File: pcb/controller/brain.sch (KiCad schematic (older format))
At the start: 0 parts

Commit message: designed v0.1 of brain board
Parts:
- added C1, C2, C3, C4, C5: 1uF, Capacitors_SMD:C_0603_HandSoldering, symbol C
- added GND1, Mode1, RX1, Reset1, TX1: TP, Measurement_Points:Measurement_Point_Round-SMD-Pad_Small, symbol TEST
- added J1: CONN_02X08, Pin_Headers:Pin_Header_Straight_2x08_Pitch2.54mm_SMD, symbol CONN_02X08
- added J10, J11, J12, J13, J14, J15, J16, J17, J18, J19, J20, J21, J22, J23, J24, J25, J26, J27, J28, J29, J30, J31, J32, J33, J34, J35, J36, J37, J38, J39, J40, J41, J42, J43, J44, J45, J46, J5, J6, J7, J8, J9: break, breakaway:0.35mil_square, symbol TEST_1P
- added J2, J3, J4: CONN_01X08, Pin_Headers:Pin_Header_Straight_1x08_Pitch2.54mm_SMD_Pin1Right, symbol CONN_01X08
- added J47, J48, J49: CONN_01X01, SMD_Packages:1Pin, symbol CONN_01X01
- added Q1, Q10, Q11, Q12, Q13, Q14, Q15, Q16, Q17, Q18, Q19, Q2, Q20, Q21, Q22, Q23, Q24, Q25, Q26, Q27, Q28, Q29, Q3, Q30, Q31, Q32, Q4, Q5, Q6, Q7, Q8, Q9: A09T, TO_SOT_Packages_SMD:SOT-23, symbol Q_NMOS_GSD
- added R1, R2: 1k, Resistors_SMD:R_0603_HandSoldering, symbol R
- added U1, U2, U3, U4: 74HC595, Housings_SOIC:SOIC-16_3.9x9.9mm_Pitch1.27mm, symbol 74HC595
- added U5: ESP-12E, ESP8266:ESP-12E_SMD, symbol ESP-12E
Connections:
- new net: R1.1, Reset1.1, U5.1 (REST)
- new net: Mode1.1, R2.1, U5.12 (GPIO0)
- new net: RX1.1, U5.15 (RXD)
- new net: TX1.1, U5.16 (TXD)
- new net: Q10.1 (G), U2.1 (QB)
- new net: Q9.1 (G), U2.15 (QA)
- new net: Q11.1 (G), U2.2 (QC)
- new net: Q12.1 (G), U2.3 (QD)
- new net: Q13.1 (G), U2.4 (QE)
- new net: Q14.1 (G), U2.5 (QF)
- new net: Q15.1 (G), U2.6 (QG)
- new net: Q16.1 (G), U2.7 (QH)
- new net: J21.1, J22.1, U2.9 (~QH), U3.14 (SER)
- new net: Q18.1 (G), U3.1 (QB)
- new net: Q17.1 (G), U3.15 (QA)
- new net: Q19.1 (G), U3.2 (QC)
- new net: Q20.1 (G), U3.3 (QD)
- new net: Q21.1 (G), U3.4 (QE)
- new net: Q22.1 (G), U3.5 (QF)
- new net: Q23.1 (G), U3.6 (QG)
- new net: Q24.1 (G), U3.7 (QH)
- new net: J33.1, J34.1, U3.9 (~QH), U4.14 (SER)
- new net: Q26.1 (G), U4.1 (QB)
- new net: Q25.1 (G), U4.15 (QA)
- new net: Q27.1 (G), U4.2 (QC)
- new net: Q28.1 (G), U4.3 (QD)
- new net: Q29.1 (G), U4.4 (QE)
- new net: Q30.1 (G), U4.5 (QF)
- new net: Q31.1 (G), U4.6 (QG)
- new net: Q32.1 (G), U4.7 (QH)
- new net: J43.1, U4.9 (~QH)
- new net: Q2.1 (G), U1.1 (QB)
- new net: Q1.1 (G), U1.15 (QA)
- new net: Q3.1 (G), U1.2 (QC)
- new net: Q4.1 (G), U1.3 (QD)
- new net: Q5.1 (G), U1.4 (QE)
- new net: Q6.1 (G), U1.5 (QF)
- new net: Q7.1 (G), U1.6 (QG)
- new net: Q8.1 (G), U1.7 (QH)
- new net +12V: J1.1 (P1), J1.2 (P2), J47.1 (P1)
- new net ADC_RCLK: J11.1, J12.1, J23.1, J24.1, J35.1, J36.1, J44.1, U2.12 (RCLK), U3.12 (RCLK), U4.12 (RCLK), U5.6 (GPIO12)
- new net CLK: J1.7 (P7), J13.1, J14.1, J25.1, J26.1, J37.1, J38.1, J45.1, U1.11 (SRCLK), U2.11 (SRCLK), U3.11 (SRCLK), U4.11 (SRCLK), U5.22 (SCLK)
- new net GND: C1.1, C2.1, C3.1, C4.1, C5.1, GND1.1, J1.3 (P3), J1.4 (P4), J15.1, J16.1, J19.1, J20.1, J27.1, J28.1, J31.1, J32.1, J39.1, J40.1, J42.1, J46.1, J49.1 (P1), J7.1, J8.1, Q1.2 (S), Q10.2 (S), Q11.2 (S), Q12.2 (S), Q13.2 (S), Q14.2 (S), Q15.2 (S), Q16.2 (S), Q17.2 (S), Q18.2 (S), Q19.2 (S), Q2.2 (S), Q20.2 (S), Q21.2 (S), Q22.2 (S), Q23.2 (S), Q24.2 (S), Q25.2 (S), Q26.2 (S), Q27.2 (S), Q28.2 (S), Q29.2 (S), Q3.2 (S), Q30.2 (S), Q31.2 (S), Q32.2 (S), Q4.2 (S), Q5.2 (S), Q6.2 (S), Q7.2 (S), Q8.2 (S), Q9.2 (S), U1.13 (G), U1.8 (GND), U2.13 (G), U2.8 (GND), U3.13 (G), U3.8 (GND), U4.13 (G), U4.8 (GND)
- new net MISO: J1.6 (P6), U5.18 (MISO)
- new net MOSI: J10.1, J9.1, U1.14 (SER), U2.14 (SER), U5.21 (MOSI)
- new net N_ADC0: J2.1 (P1), Q9.3 (D)
- new net N_ADC1: J2.2 (P2), Q10.3 (D)
- new net N_ADC10: J3.3 (P3), Q19.3 (D)
- new net N_ADC11: J3.4 (P4), Q20.3 (D)
- new net N_ADC12: J3.5 (P5), Q21.3 (D)
- new net N_ADC13: J3.6 (P6), Q22.3 (D)
- new net N_ADC14: J3.7 (P7), Q23.3 (D)
- new net N_ADC15: J3.8 (P8), Q24.3 (D)
- new net N_ADC16: J4.1 (P1), Q25.3 (D)
- new net N_ADC17: J4.2 (P2), Q26.3 (D)
- new net N_ADC18: J4.3 (P3), Q27.3 (D)
- new net N_ADC19: J4.4 (P4), Q28.3 (D)
- new net N_ADC2: J2.3 (P3), Q11.3 (D)
- new net N_ADC20: J4.5 (P5), Q29.3 (D)
- new net N_ADC21: J4.6 (P6), Q30.3 (D)
- new net N_ADC22: J4.7 (P7), Q31.3 (D)
- new net N_ADC23: J4.8 (P8), Q32.3 (D)
- new net N_ADC3: J2.4 (P4), Q12.3 (D)
- new net N_ADC4: J2.5 (P5), Q13.3 (D)
- new net N_ADC5: J2.6 (P6), Q14.3 (D)
- new net N_ADC6: J2.7 (P7), Q15.3 (D)
- new net N_ADC7: J2.8 (P8), Q16.3 (D)
- new net N_ADC8: J3.1 (P1), Q17.3 (D)
- new net N_ADC9: J3.2 (P2), Q18.3 (D)
- new net N_LOAD: J1.8 (P8), U5.10 (GPIO15)
- new net N_START0: J1.9 (P9), Q1.3 (D)
- new net N_START1: J1.10 (P10), Q2.3 (D)
- new net N_START2: J1.11 (P11), Q3.3 (D)
- new net N_START3: J1.12 (P12), Q4.3 (D)
- new net N_START4: J1.13 (P13), Q5.3 (D)
- new net N_START5: J1.14 (P14), Q6.3 (D)
- new net N_START6: J1.15 (P15), Q7.3 (D)
- new net N_START7: J1.16 (P16), Q8.3 (D)
- new net START_RCLK: U1.12 (RCLK), U5.7 (GPIO13)
- new net VCC: C1.2, C2.2, C3.2, C4.2, C5.2, J1.5 (P5), J17.1, J18.1, J29.1, J30.1, J41.1, J48.1 (P1), J5.1, J6.1, R1.2, R2.2, U1.10 (SRCLR), U1.16 (VCC), U2.10 (SRCLR), U2.16 (VCC), U3.10 (SRCLR), U3.16 (VCC), U4.10 (SRCLR), U4.16 (VCC)
- no-connect marks 0 -> 13

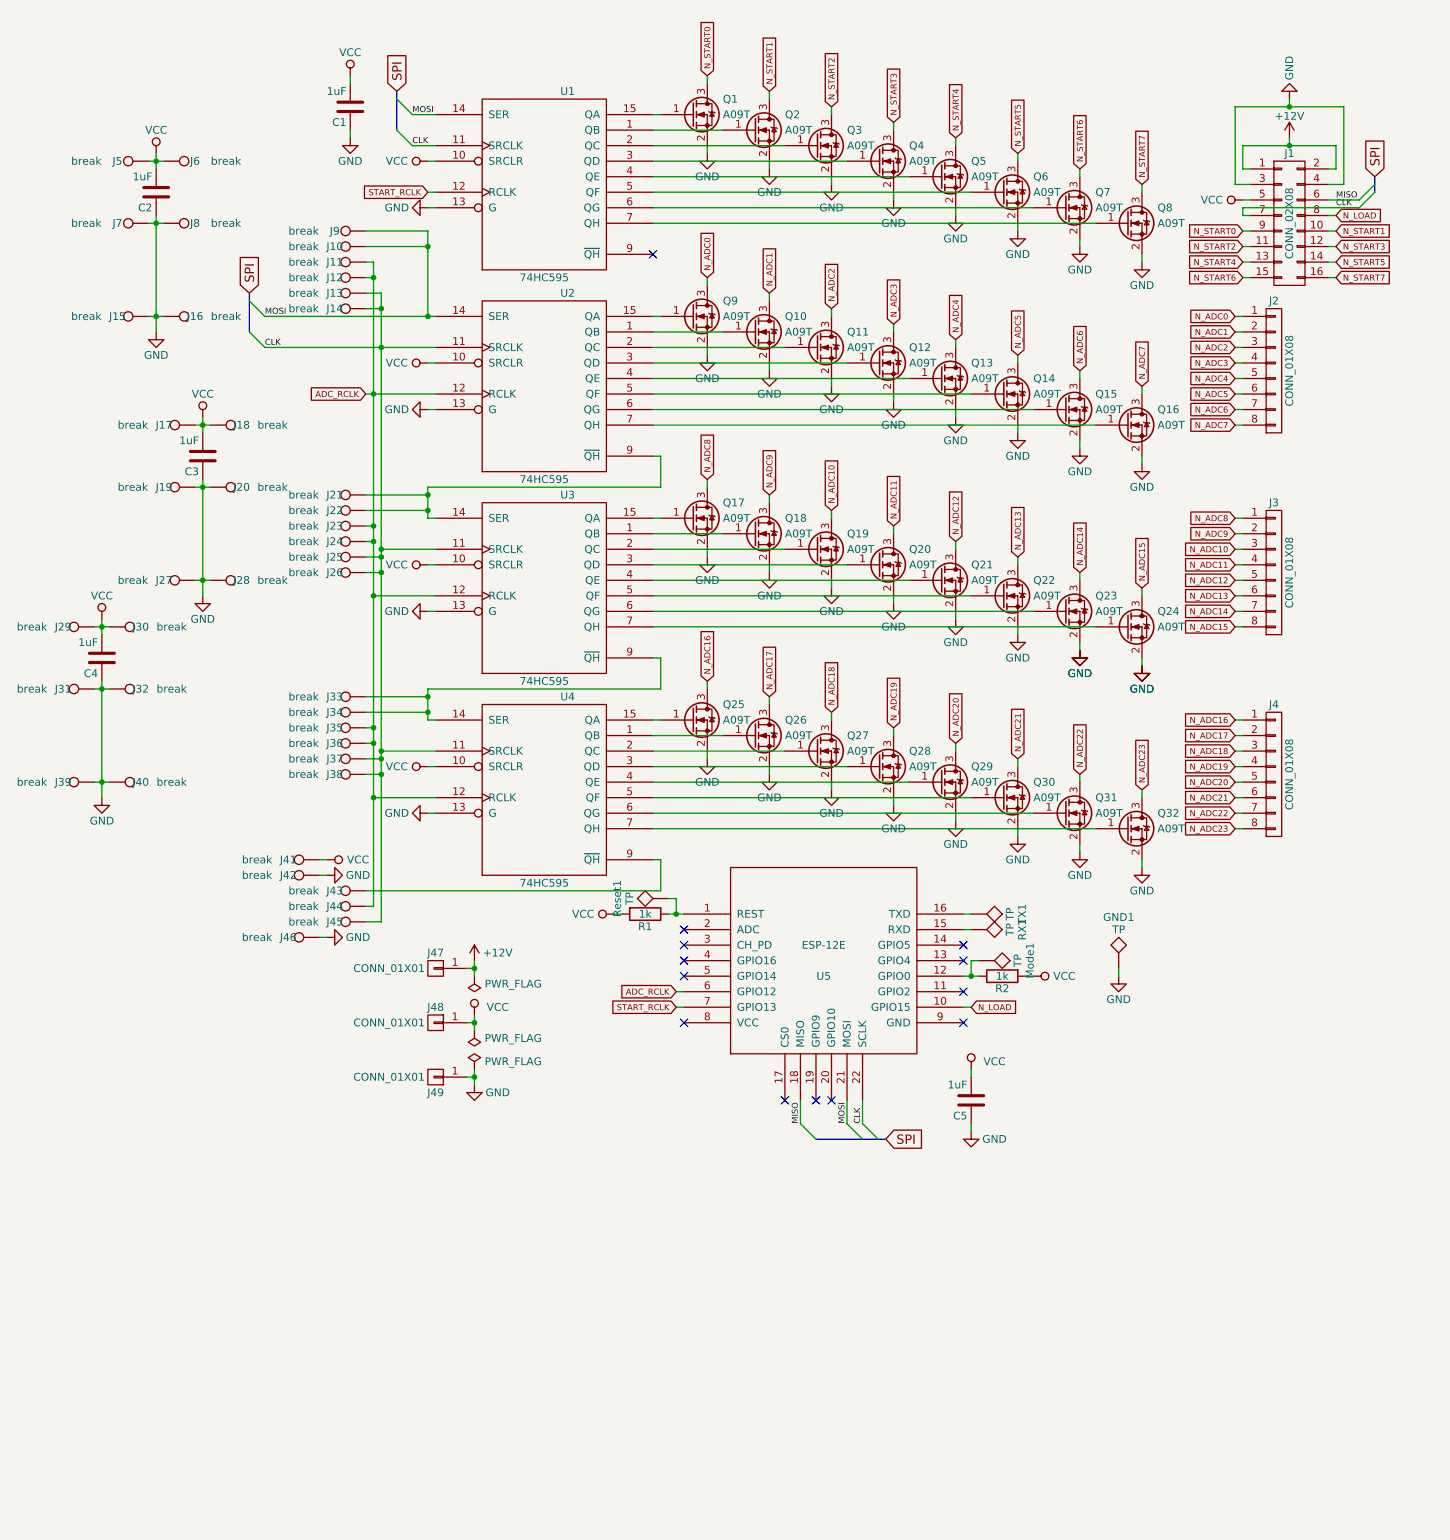
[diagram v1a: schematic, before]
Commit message: begins to further develop controller
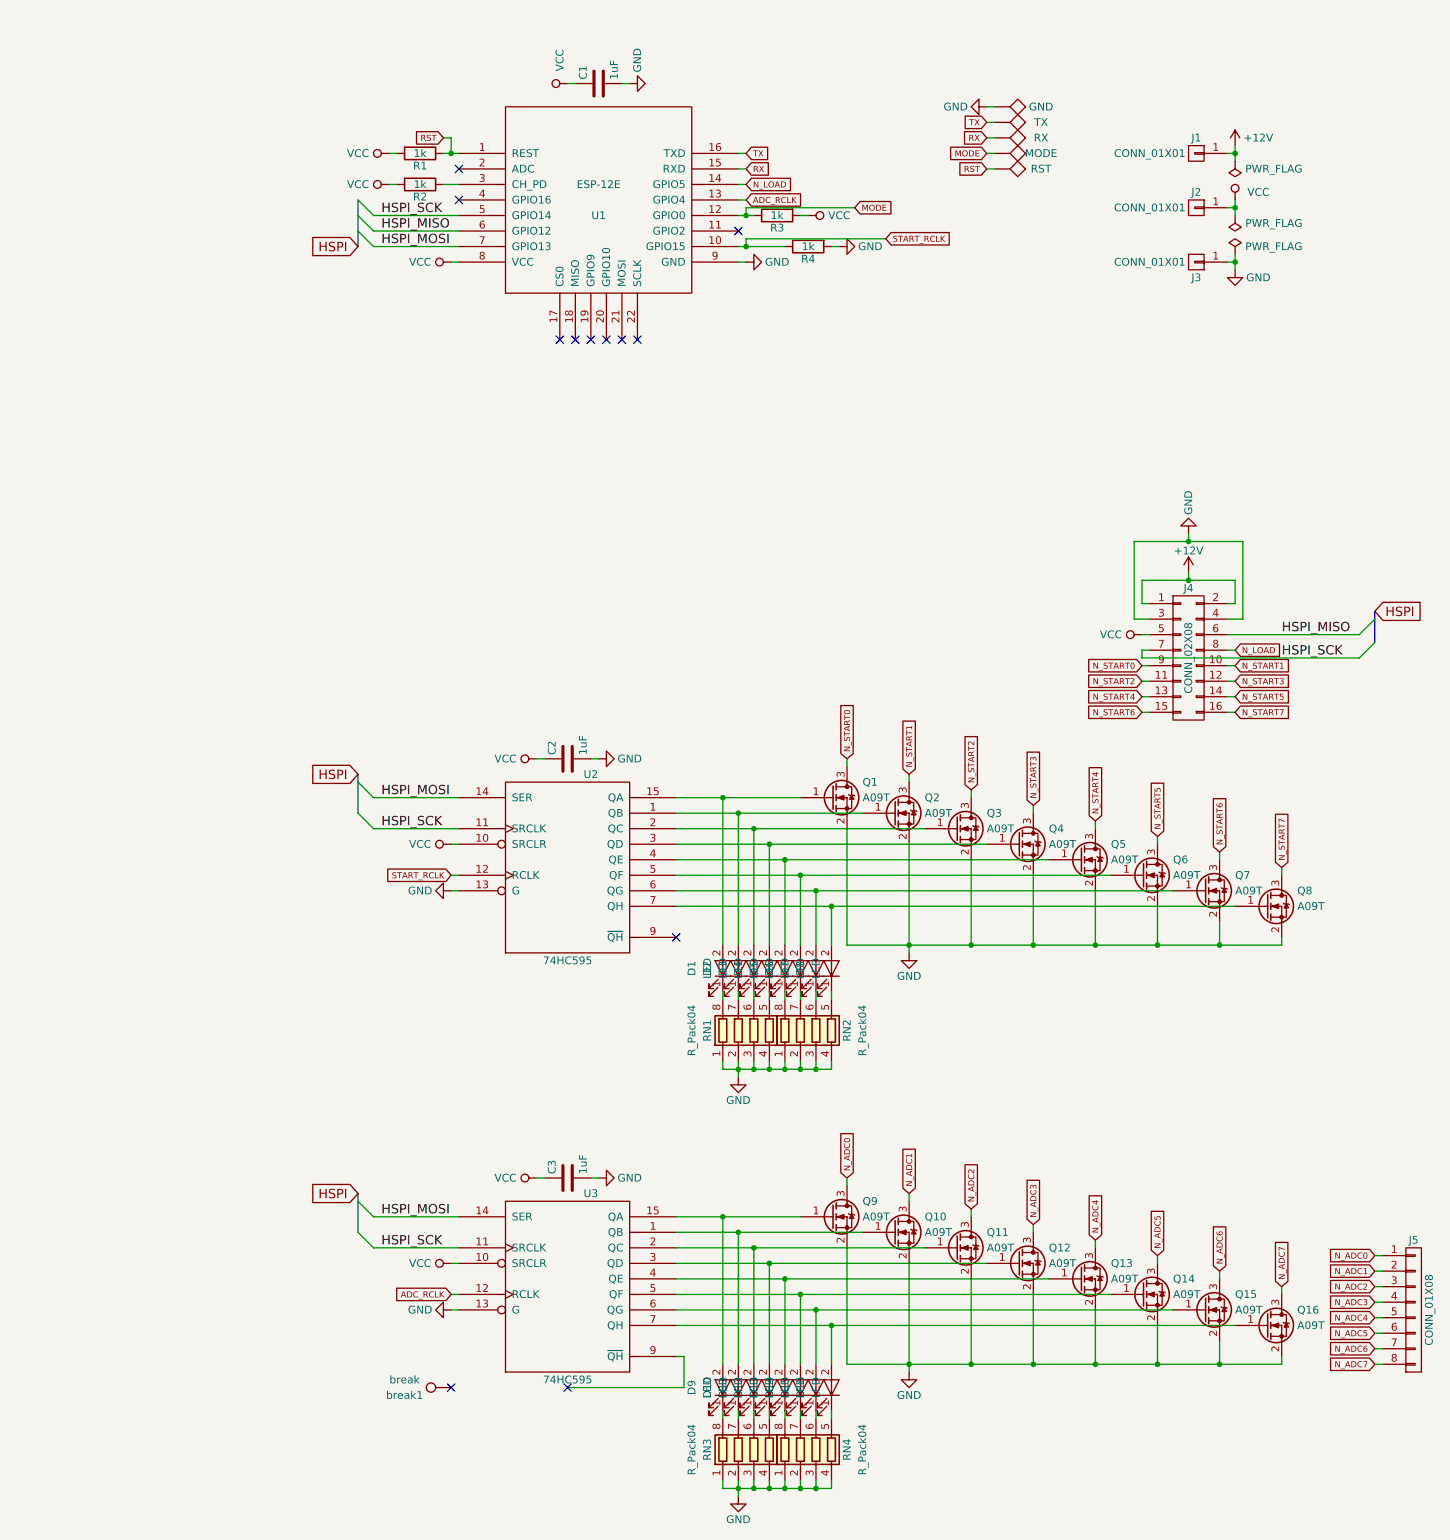
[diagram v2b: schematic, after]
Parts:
- removed C2, C4: 1uF, Capacitors_SMD:C_0603_HandSoldering, symbol C
- removed J10, J11, J12, J13, J14, J15, J16, J17, J18, J19, J20, J21, J22, J23, J24, J25, J26, J27, J28, J29, J30, J31, J32, J33, J34, J35, J36, J37, J38, J39, J40, J41, J42, J43, J44, J45, J46, J5, J6, J7, J8, J9: break, breakaway:0.35mil_square, symbol TEST_1P
- removed J3, J4: CONN_01X08, Pin_Headers:Pin_Header_Straight_1x08_Pitch2.54mm_SMD_Pin1Right, symbol CONN_01X08
- removed Q17, Q18, Q19, Q20, Q21, Q22, Q23, Q24, Q25, Q26, Q27, Q28, Q29, Q30, Q31, Q32: A09T, TO_SOT_Packages_SMD:SOT-23, symbol Q_NMOS_GSD
- removed U2, U4: 74HC595, Housings_SOIC:SOIC-16_3.9x9.9mm_Pitch1.27mm, symbol 74HC595
- added D1, D10, D11, D12, D13, D14, D15, D16, D2, D3, D4, D5, D6, D7, D8, D9: LED, LEDs:LED_0603, symbol LED
- added R2, R4: 1k, Resistors_SMD:R_0603_HandSoldering, symbol R
- added RN1, RN2, RN3, RN4: R_Pack04, Resistors_SMD:R_Array_Convex_4x0603, symbol R_Pack04
- added break1: break, symbol TEST_1P
- J4: renamed from J1; footprint Pin_Headers:Pin_Header_Straight_2x08_Pitch2.54mm_SMD -> Connectors:IDC_Header_SMD_16pins
- TP1: renamed from GND1; value TP -> GND
- TP2: renamed from TX1; value TP -> TX
- TP3: renamed from RX1; value TP -> RX
- TP4: renamed from Mode1; value TP -> MODE
- TP5: renamed from Reset1; value TP -> RST
- renumbered C5 to C1, C1 to C2, J47 to J1, J48 to J2, J49 to J3, J2 to J5, R2 to R3, U5 to U1, U1 to U2
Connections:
- net ADC_RCLK: now also U1.13 (GPIO4); no longer U1.6 (GPIO12)
- net GND: now also C1.2, C2.2, C3.2, U1.9 (GND), R4.2, RN1.1 (R1.1), RN1.2 (R2.1), RN1.3 (R3.1), RN1.4 (R4.1), RN2.1 (R1.1), RN2.2 (R2.1), RN2.3 (R3.1), RN2.4 (R4.1), RN3.1 (R1.1), RN3.2 (R2.1), RN3.3 (R3.1), RN3.4 (R4.1), RN4.1 (R1.1), RN4.2 (R2.1), RN4.3 (R3.1), RN4.4 (R4.1); no longer C1.1, C2.1, C3.1
- net N_LOAD: now also U1.14 (GPIO5); no longer U1.10 (GPIO15)
- net START_RCLK: now also U1.10 (GPIO15), R4.1; no longer U1.7 (GPIO13)
- net VCC: now also C1.1, C2.1, C3.1, U1.8 (VCC), R2.2; no longer C1.2, C2.2, C3.2
- net RST: now reaches R1.1, TP5.1, U1.1 (REST)
- net MODE: now reaches R3.1, TP4.1, U1.12 (GPIO0)
- net RX: now reaches TP3.1, U1.15 (RXD)
- net TX: now reaches TP2.1, U1.16 (TXD)
- net at U1.3 (CH_PD): now also R2.1
- net HSPI_SCK: now reaches U1.5 (GPIO14)
- net HSPI_SCK: now also J4.7 (P7), U2.11 (SRCLK), U3.11 (SRCLK)
- net at Q10.1 (G): now also U3.1 (QB), D10.2 (A)
- net at Q9.1 (G): now also U3.15 (QA), D9.2 (A)
- net at Q11.1 (G): now also U3.2 (QC), D11.2 (A)
- net at Q12.1 (G): now also U3.3 (QD), D12.2 (A)
- net at Q13.1 (G): now also U3.4 (QE), D13.2 (A)
- net at Q14.1 (G): now also U3.5 (QF), D14.2 (A)
- net at Q15.1 (G): now also U3.6 (QG), D15.2 (A)
- net at Q16.1 (G): now also U3.7 (QH), D16.2 (A)
- net HSPI_MOSI: now reaches U3.14 (SER)
- net HSPI_MOSI: now also U1.7 (GPIO13), U2.14 (SER)
- net at Q2.1 (G), U2.1 (QB): now also D2.2 (A)
- net at Q1.1 (G), U2.15 (QA): now also D1.2 (A)
- net at Q3.1 (G), U2.2 (QC): now also D3.2 (A)
- net at Q4.1 (G), U2.3 (QD): now also D4.2 (A)
- net at Q5.1 (G), U2.4 (QE): now also D5.2 (A)
- net at Q6.1 (G), U2.5 (QF): now also D6.2 (A)
- net at Q7.1 (G), U2.6 (QG): now also D7.2 (A)
- net at Q8.1 (G), U2.7 (QH): now also D8.2 (A)
- removed net CLK: J4.7 (P7), U1.22 (SCLK), U2.11 (SRCLK), U3.11 (SRCLK)
- net MISO: no longer names the net of U1.18 (MISO)
- net MISO: no longer J4.6 (P6)
- net MOSI: no longer names the net of U1.21 (MOSI)
- net MOSI: no longer U2.14 (SER)
- new net: D4.1 (K), RN1.5 (R4.2)
- new net: D3.1 (K), RN1.6 (R3.2)
- new net: D2.1 (K), RN1.7 (R2.2)
- new net: D1.1 (K), RN1.8 (R1.2)
- new net: D8.1 (K), RN2.5 (R4.2)
- new net: D7.1 (K), RN2.6 (R3.2)
- new net: D6.1 (K), RN2.7 (R2.2)
- new net: D5.1 (K), RN2.8 (R1.2)
- new net: D12.1 (K), RN3.5 (R4.2)
- new net: D11.1 (K), RN3.6 (R3.2)
- new net: D10.1 (K), RN3.7 (R2.2)
- new net: D9.1 (K), RN3.8 (R1.2)
- new net: D16.1 (K), RN4.5 (R4.2)
- new net: D15.1 (K), RN4.6 (R3.2)
- new net: D14.1 (K), RN4.7 (R2.2)
- new net: D13.1 (K), RN4.8 (R1.2)
- new net HSPI_MISO: J4.6 (P6), U1.6 (GPIO12)
- no-connect marks 13 -> 12
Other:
- moved on the sheet: C1, C2, J1, J2, J3, J4, J5, Q1, Q2, Q3, Q4, Q5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
